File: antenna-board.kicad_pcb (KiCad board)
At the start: 2 copper layers, 42.4 x 42.4 mm, 2 parts, among them J1 Conn_01x01, U1 U.FLport

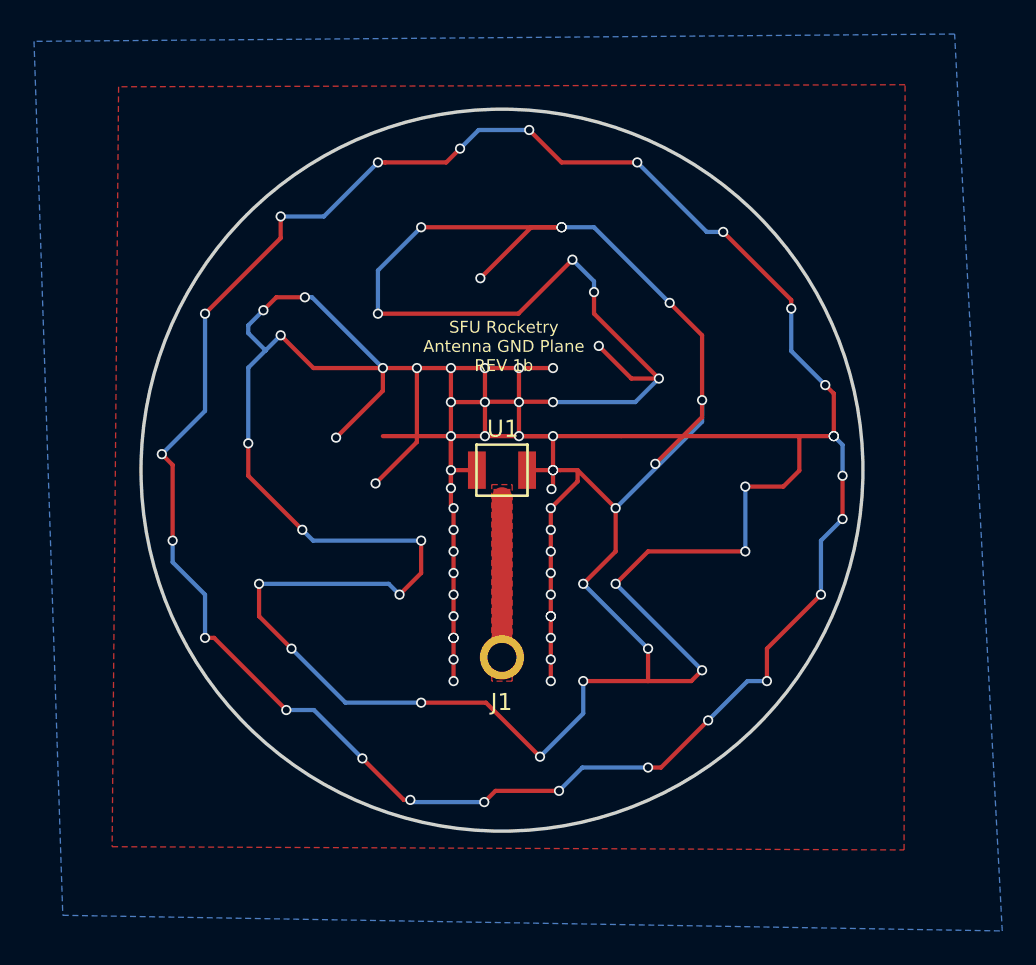
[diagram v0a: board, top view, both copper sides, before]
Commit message: Fixed Vias
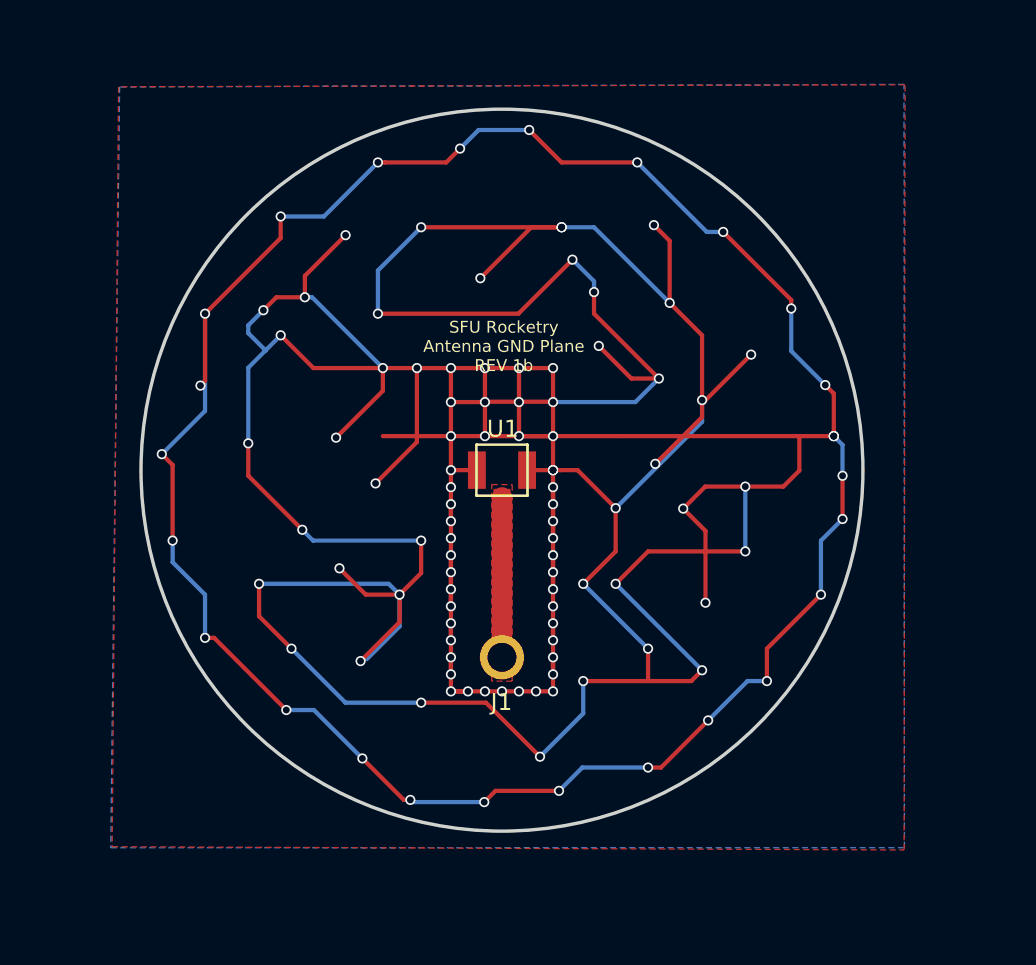
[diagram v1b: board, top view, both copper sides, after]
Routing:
- net GNDREF: track 447.4 -> 508.9 mm, vias 97 -> 114
